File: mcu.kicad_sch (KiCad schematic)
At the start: 11 parts, among them J1 USB4105-GF-A, Q2 BC847BDW1, U1 ESP32-C6-MINI-1, U4 FT231XQ

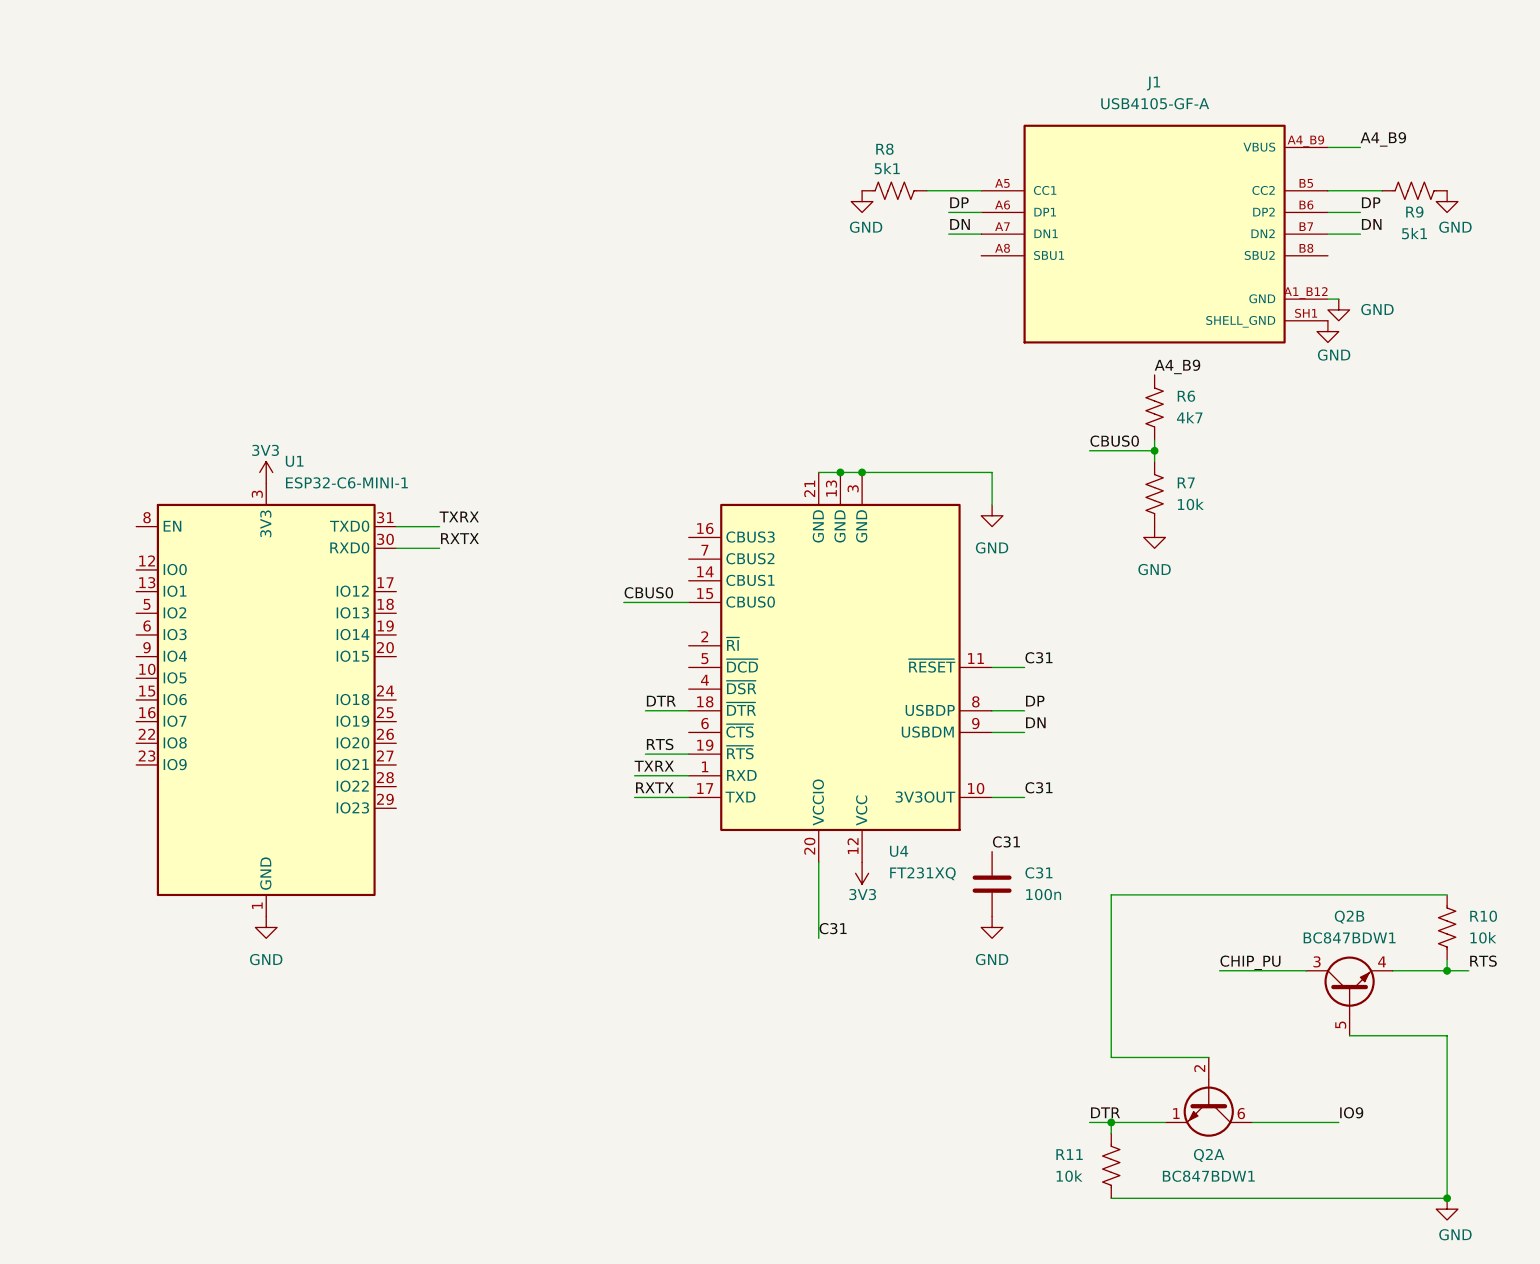
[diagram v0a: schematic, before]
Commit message: added switched
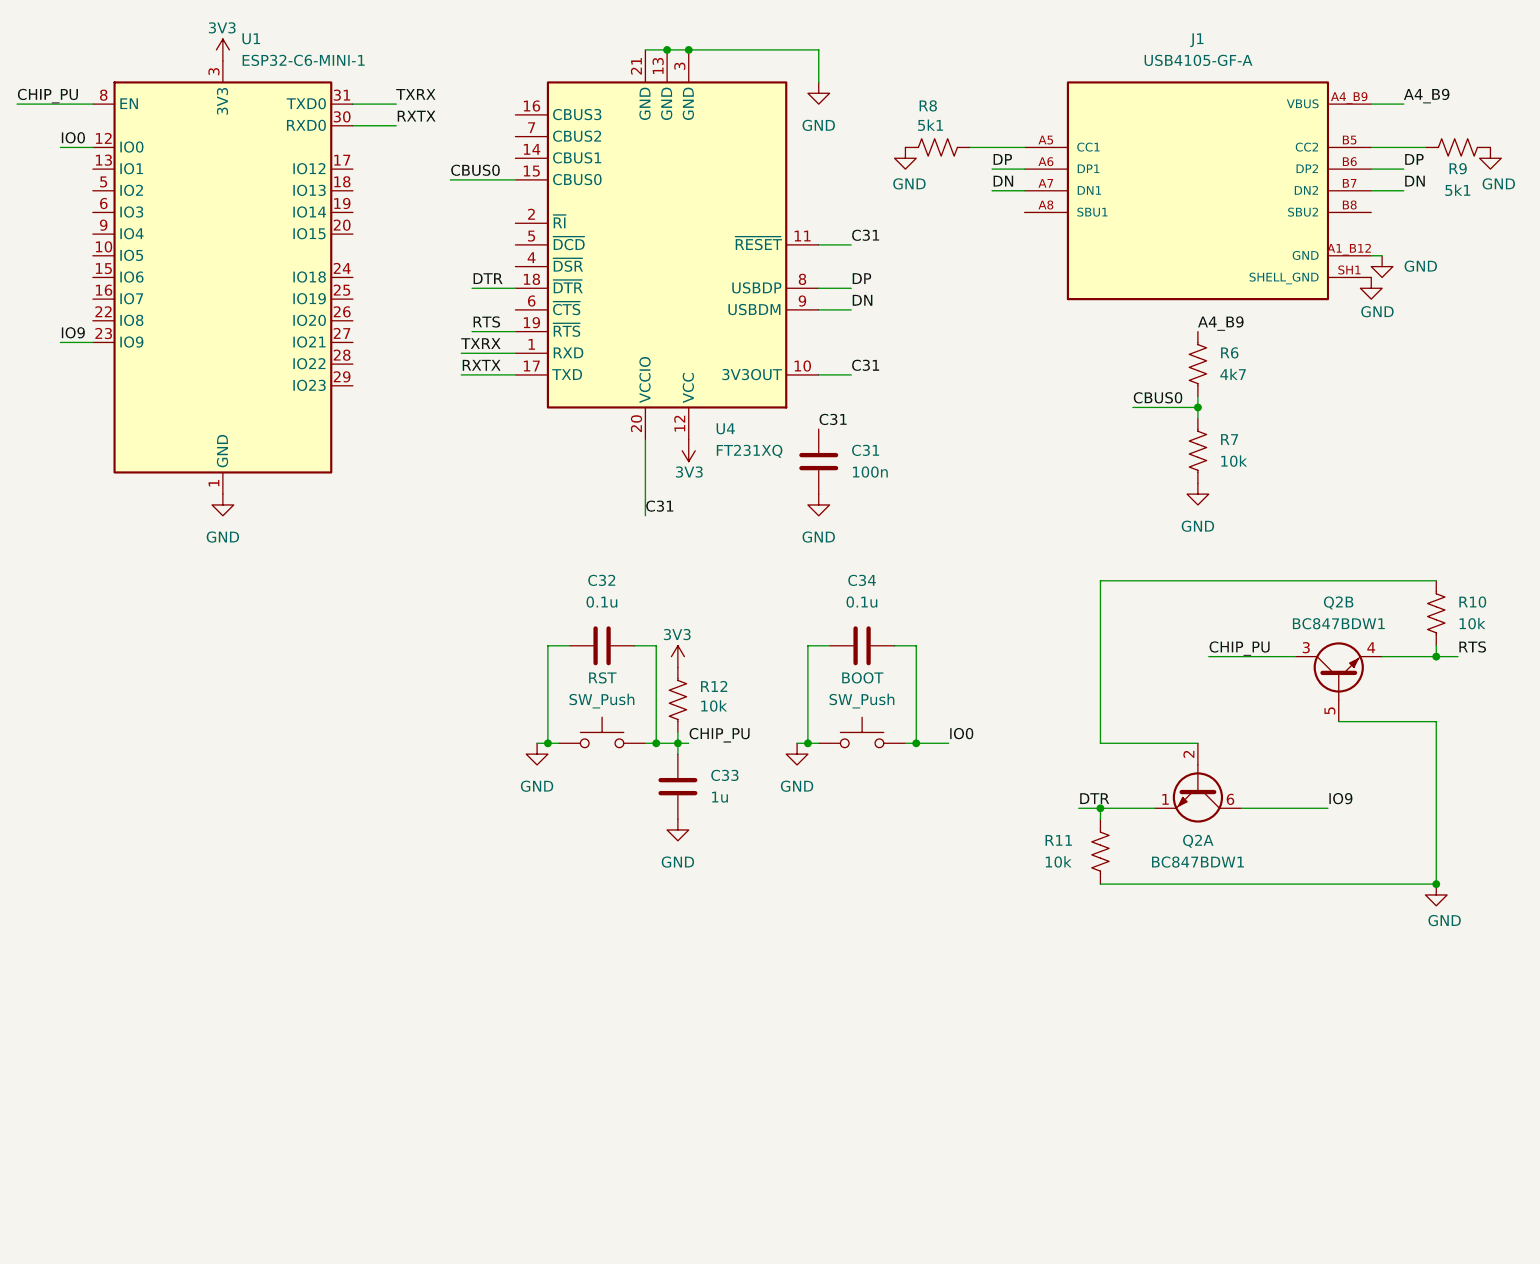
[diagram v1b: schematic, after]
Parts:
- added BOOT, RST: SW_Push, symbol Switch:SW_Push
- added C32, C34: 0.1u, symbol Device:C
- added C33: 1u, symbol Device:C
- added R12: 10k, symbol Device:R_US
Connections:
- net 3V3: now also R12.1
- net CHIP_PU: now also U1.8 (EN), C32.1, C33.2, R12.2, RST.2
- net GND: now also BOOT.1, C32.2, C33.1, C34.2, RST.1
- net IO9: now also U1.23 (IO9)
- net IO0: now reaches U1.12 (IO0)
- net IO0: now also BOOT.2, C34.1
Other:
- moved on the sheet: C31, J1, Q2A, Q2B, R10, R11, R6, R7, R8, R9, U1, U4
